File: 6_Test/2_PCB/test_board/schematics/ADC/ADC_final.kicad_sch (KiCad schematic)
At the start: 26 parts, among them J10 Chip_AVSS_GND_Jumpers, J5 Chip_VDD_Jumpers, J6 BNC_Odd, J7 BNC_Even, J8 BNC_Jumpers, J9 Analog_Input_Jumpers

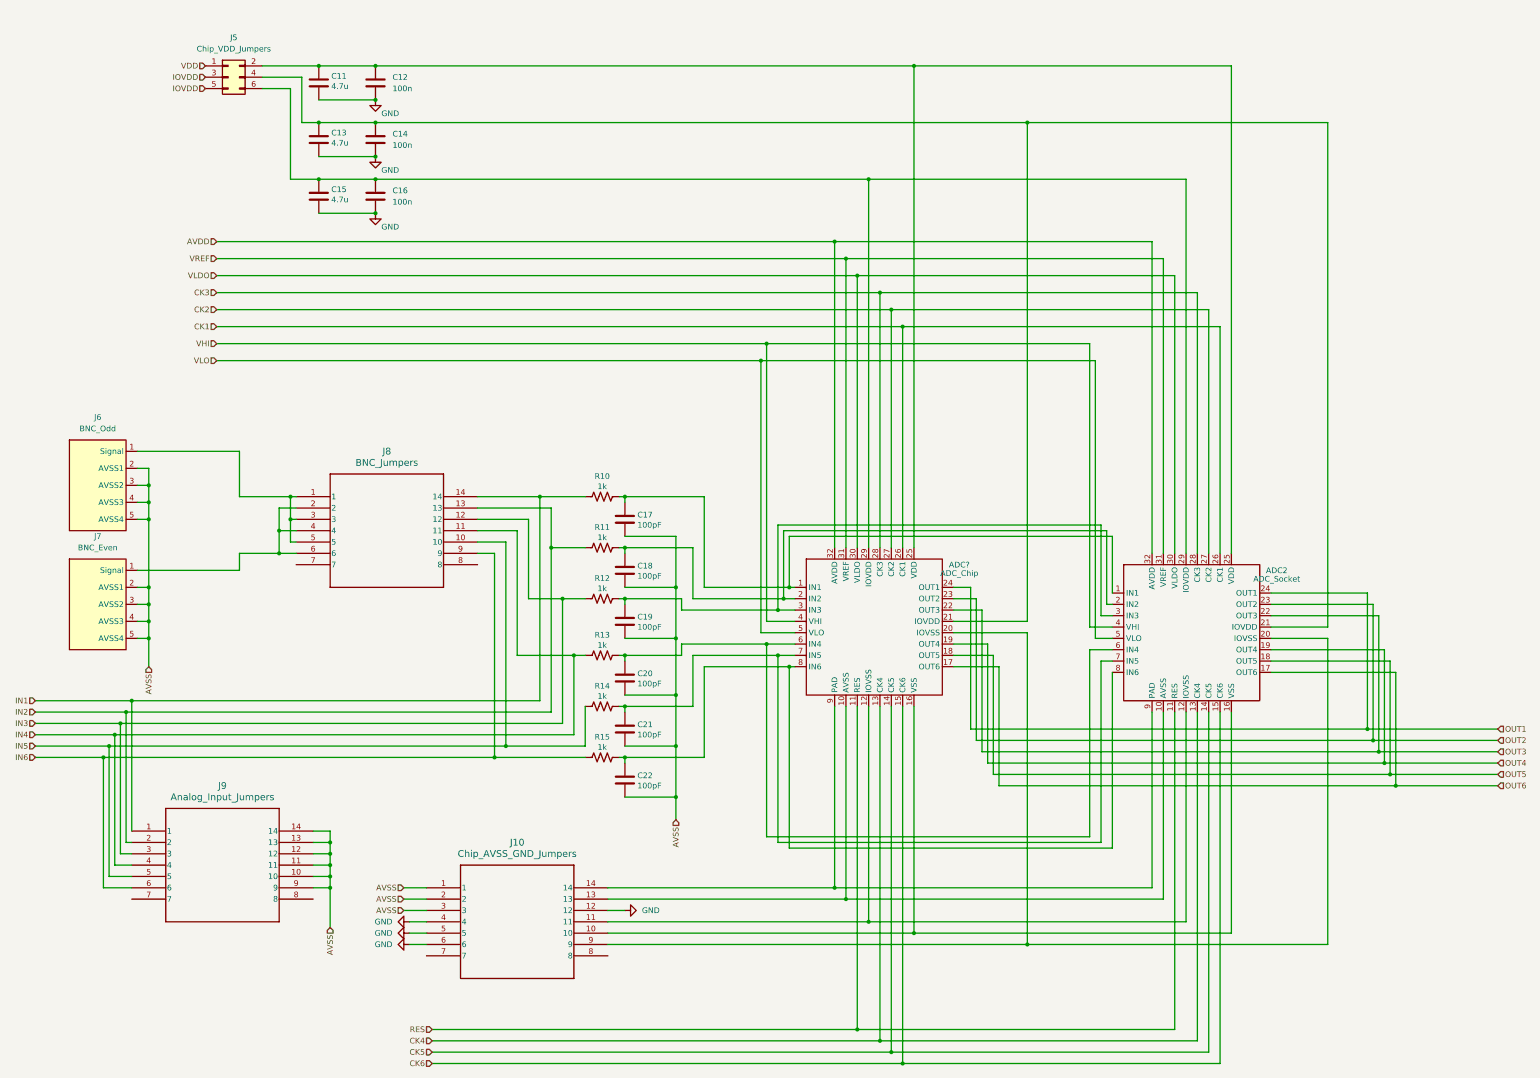
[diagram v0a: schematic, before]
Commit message: final draft of board, revision 2
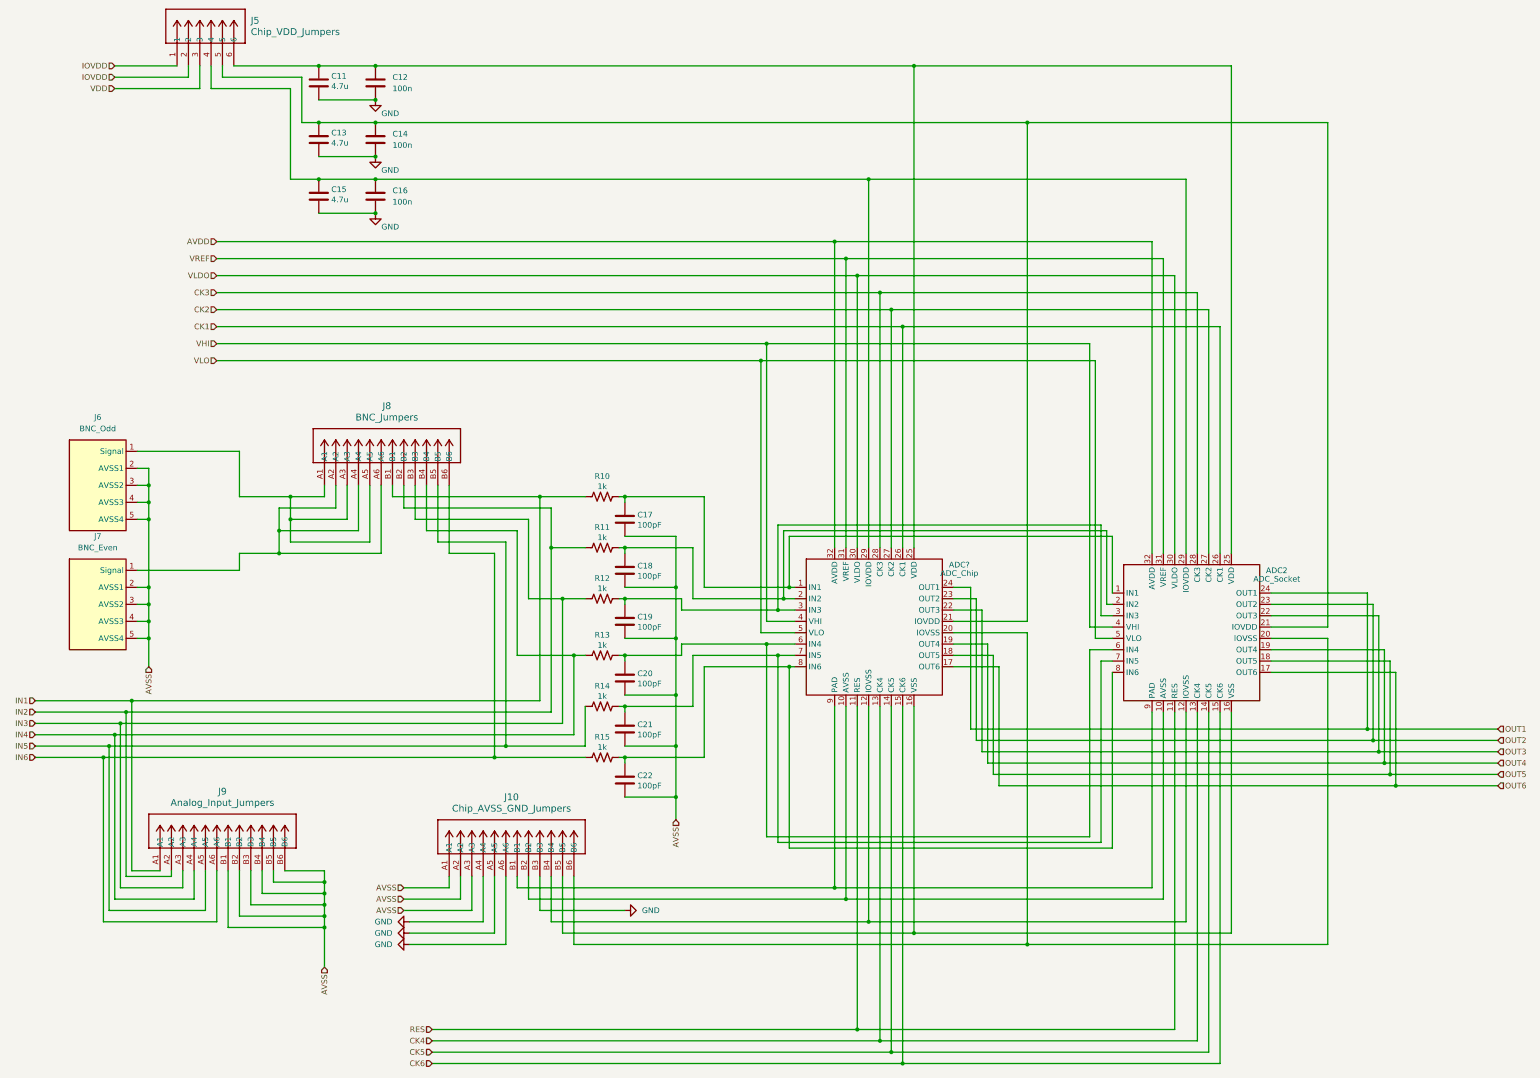
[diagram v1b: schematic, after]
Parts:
- removed J10: Chip_AVSS_GND_Jumpers, ECE628_lib:6x2header, symbol 6x2Header:TSW-107-07-F-D
- removed J5: Chip_VDD_Jumpers, Connector_PinHeader_2.54mm:PinHeader_2x03_P2.54mm_Vertical, symbol Connector_Generic:Conn_02x03_Odd_Even
- removed J8: BNC_Jumpers, TSW-107-07-G-D_SAI, symbol 6x2Header:TSW-107-07-F-D
- removed J9: Analog_Input_Jumpers, TSW-107-07-G-D_SAI, symbol 6x2Header:TSW-107-07-F-D
- added J10: Chip_AVSS_GND_Jumpers, CONN_713080000-SD_12_M6p10_MOL, symbol 2x6Header:15910120
- added J5: Chip_VDD_Jumpers, CONN6_M20-8760342_HRW, symbol 2x3Header:M20-8760342
- added J8: BNC_Jumpers, CONN_713080000-SD_12_M6p10_MOL, symbol 2x6Header:15910120
- added J9: Analog_Input_Jumpers, CONN_713080000-SD_12_M6p10_MOL, symbol 2x6Header:15910120
- C11, C13, C15: footprint Cap4.7uFFootprints:CAP_0603_CL10A_1P6XP8_SAM -> Capacitor_SMD:C_0603_1608Metric
- C12, C14, C16: footprint cap100nFFootprints:CAP_CL05_SAM -> Capacitor_SMD:C_0402_1005Metric
- C17, C18, C19, C20, C21, C22: footprint cap100pFFootprints:G-033_MUR -> Capacitor_SMD:C_0201_0603Metric
- R10, R11, R12, R13, R14, R15: footprint resistor1kFootprints:RC0402N_YAG -> Resistor_SMD:R_0402_1005Metric
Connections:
- net AVSS: now also J10.A1, J10.A2, J10.A3, J9.B1, J9.B2, J9.B3, J9.B4, J9.B5, J9.B6
- net GND: now also J10.A4, J10.A5, J10.A6, J10.B3
- net IN1: now also J8.B1, J9.A1
- net IN2: now also J8.B2, J9.A2
- net IN3: now also J8.B3, J9.A3
- net IN4: now also J8.B4, J9.A4
- net IN5: now also J8.B5, J9.A5
- net IN6: now also J8.B6, J9.A6
- net IOVDD: now also J5.1, J5.2
- net VDD: now also J5.3
- net at ADC2.25 (VDD), ADC?.25 (VDD), C11.1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: now also J5.6
- net at ADC2.21 (IOVDD), ADC?.21 (IOVDD), C13.1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: now also J5.5
- net at ADC2.29 (IOVDD), ADC?.29 (IOVDD), C15.1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: now also J5.4
- net at J6.1 (Signal): now also J8.A1, J8.A3, J8.A5
- net at ADC2.16 (VSS), ADC?.16 (VSS): now also J10.B5
- net at ADC2.12 (IOVSS), ADC?.12 (IOVSS): now also J10.B4
- net at ADC2.10 (AVSS), ADC?.10 (AVSS): now also J10.B2
- net at ADC2.9 (PAD), ADC?.9 (PAD): now also J10.B1
- net at ADC2.20 (IOVSS), ADC?.20 (IOVSS): now also J10.B6
- net at J7.1 (Signal): now also J8.A2, J8.A4, J8.A6
